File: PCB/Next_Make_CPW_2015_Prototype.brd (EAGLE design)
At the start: 41.6 x 36.8 mm, 10 parts

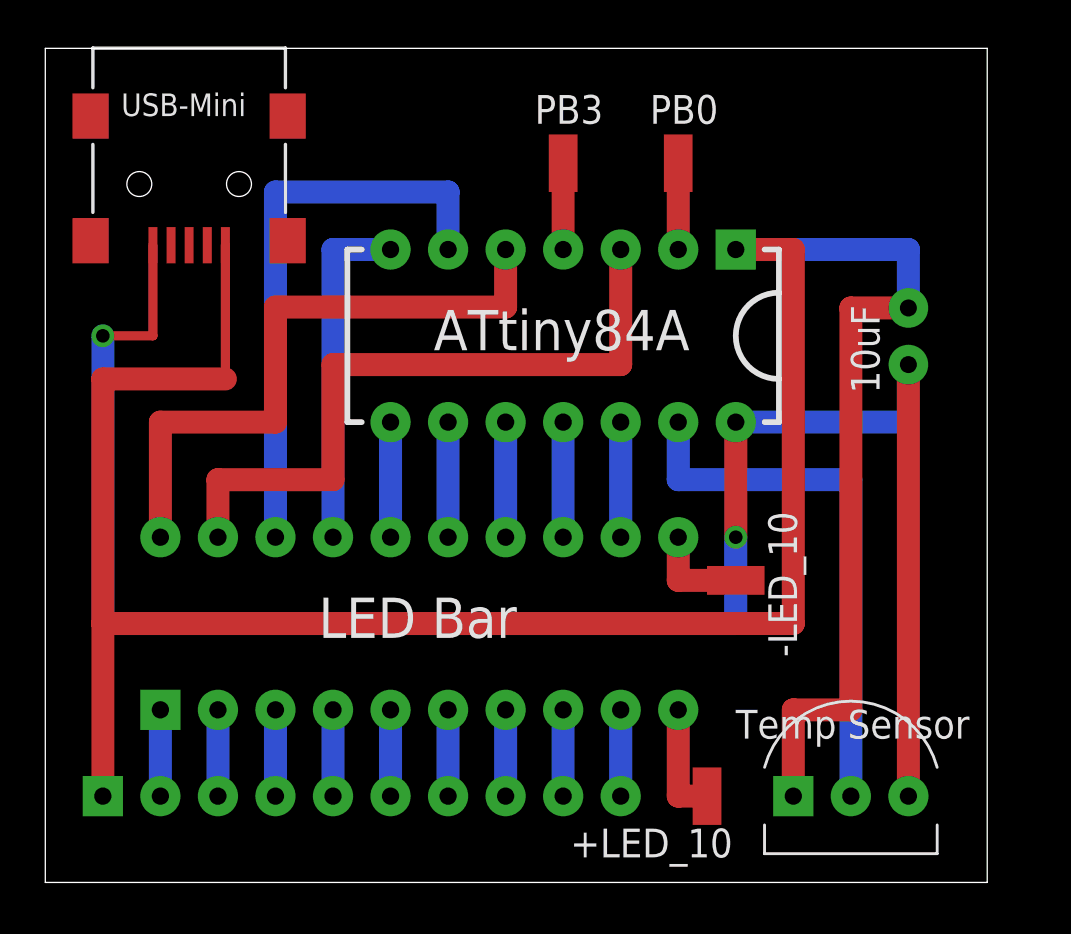
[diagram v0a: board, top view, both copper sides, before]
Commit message: final board design and updated library
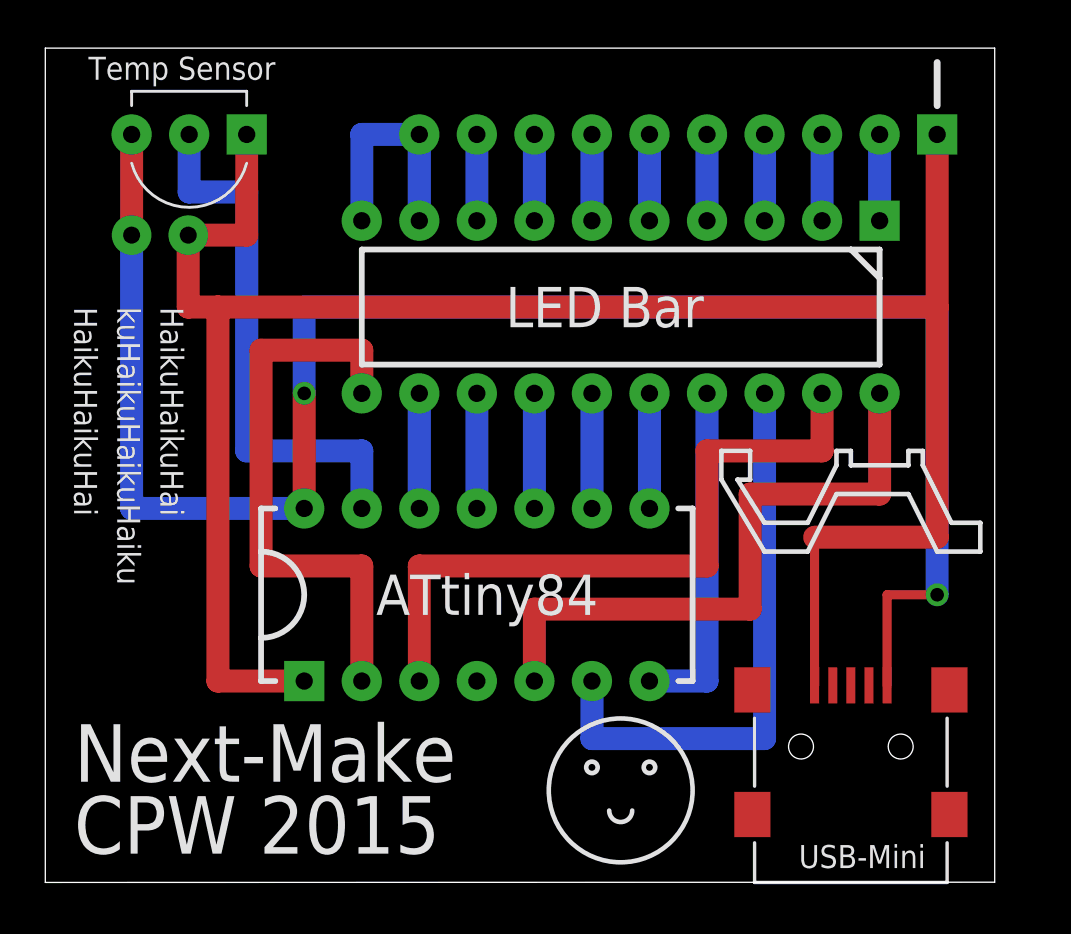
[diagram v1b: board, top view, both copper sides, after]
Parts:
- removed +LED_10, -LED_10, PB0, PB3: (no value), wirepad:SMD1,27-2,54
- moved U$1 47.0 mm to (39.4, 33.0), turned to 270 degrees
- moved U$6 47.0 mm to (35.6, 0.00), turned to 90 degrees
- moved U$4 38.4 mm to (36.8, 29.2), turned to 270 degrees
- moved U$5 37.9 mm to (8.89, 33.0), turned to 180 degrees
- moved U$2 34.8 mm to (3.81, 28.6), turned to 0 degrees
- moved U$3 22.2 mm to (26.7, 8.89), turned to 90 degrees
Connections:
- removed net N$22: PB0.1, U$3.PIN_2
- removed net N$23: PB3.1, U$3.PIN_4
- removed net N$9: U$1.PIN_10, U$4.PIN_9
- net N$20: now also U$1.PIN_10, U$4.PIN_9; no longer +LED_10.1
- net N$21: now also U$3.PIN_2; no longer -LED_10.1
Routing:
- net 5V: track 116.1 -> 93.3 mm
- net N$21: track 4.44 -> 25.4 mm
- net N$20: track 5.08 -> 10.2 mm
- net GND: track 85.0 -> 79.9 mm
- net N$9: track 3.81 -> 0.00 mm
- net N$23: track 3.81 -> 0.00 mm
- net N$22: track 3.81 -> 0.00 mm
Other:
- board size 41.6 x 36.8 mm -> 41.9 x 36.8 mm
- board text added: "ATtiny84"
- board text added: "HaikuHaikuHai"
- board text added: "kuHaikuHaikuHaiku"
- board text removed: "10uF"
- board text removed: "ATtiny84A"
